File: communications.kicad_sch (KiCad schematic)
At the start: 3 parts, among them J23 Conn_01x90_3Row_Socket

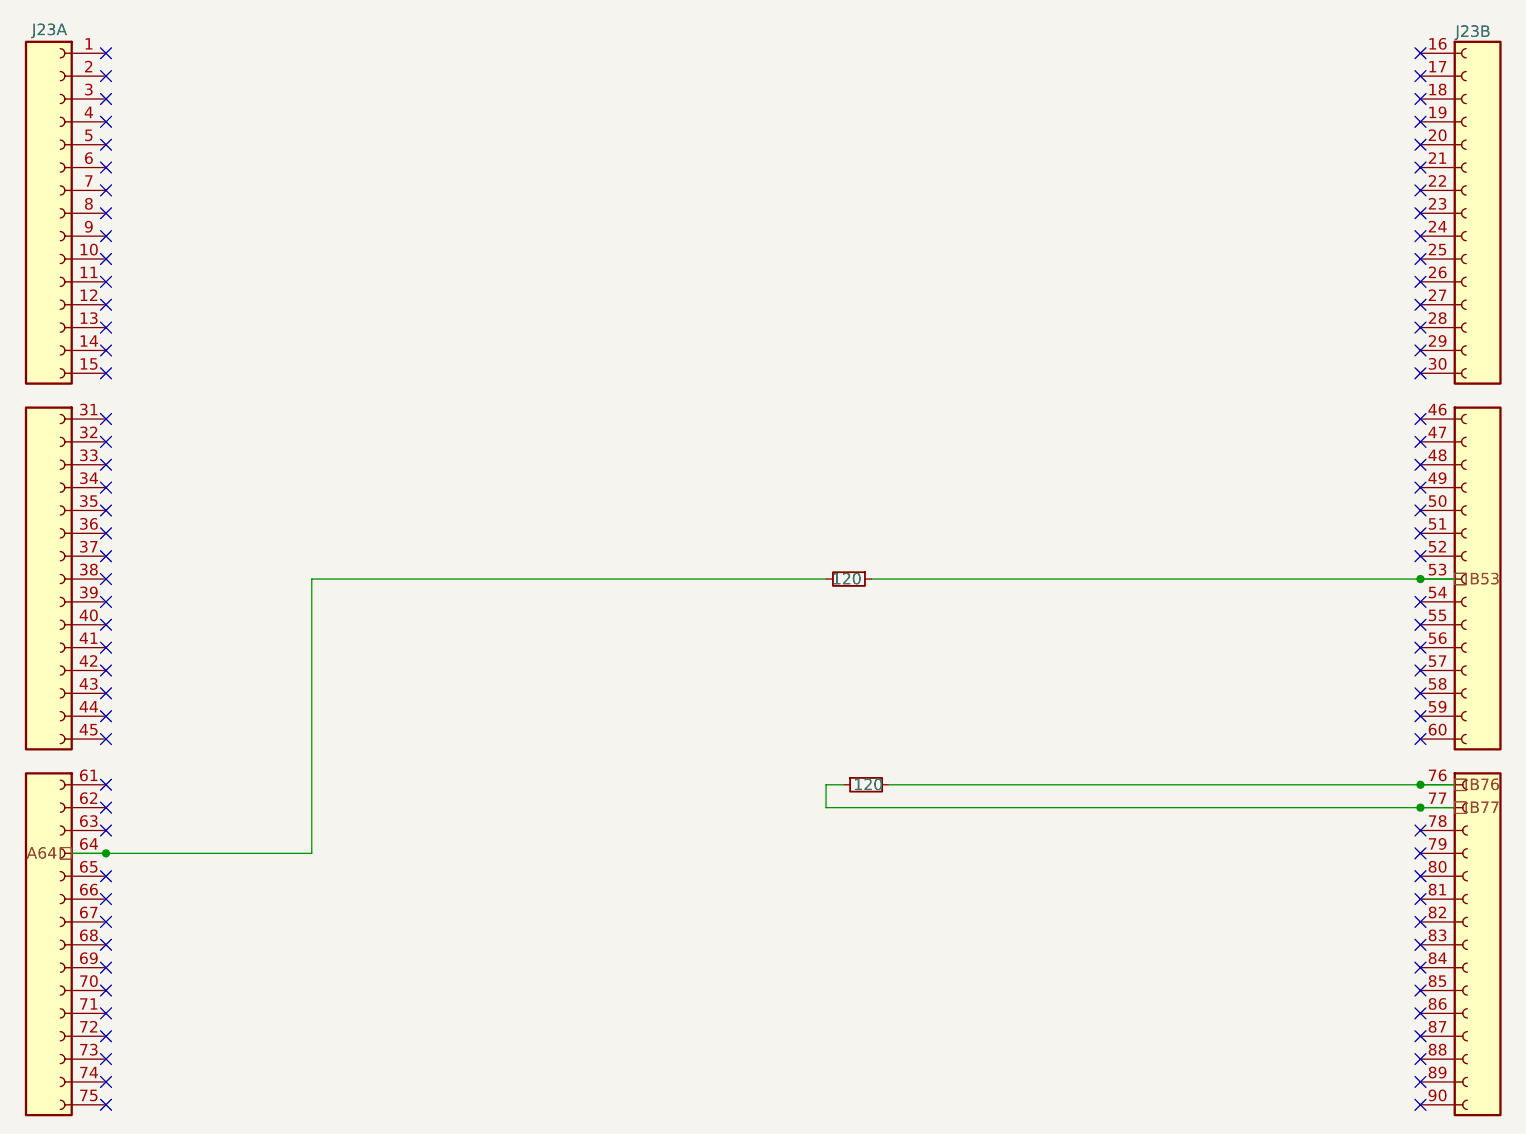
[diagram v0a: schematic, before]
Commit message: external loops
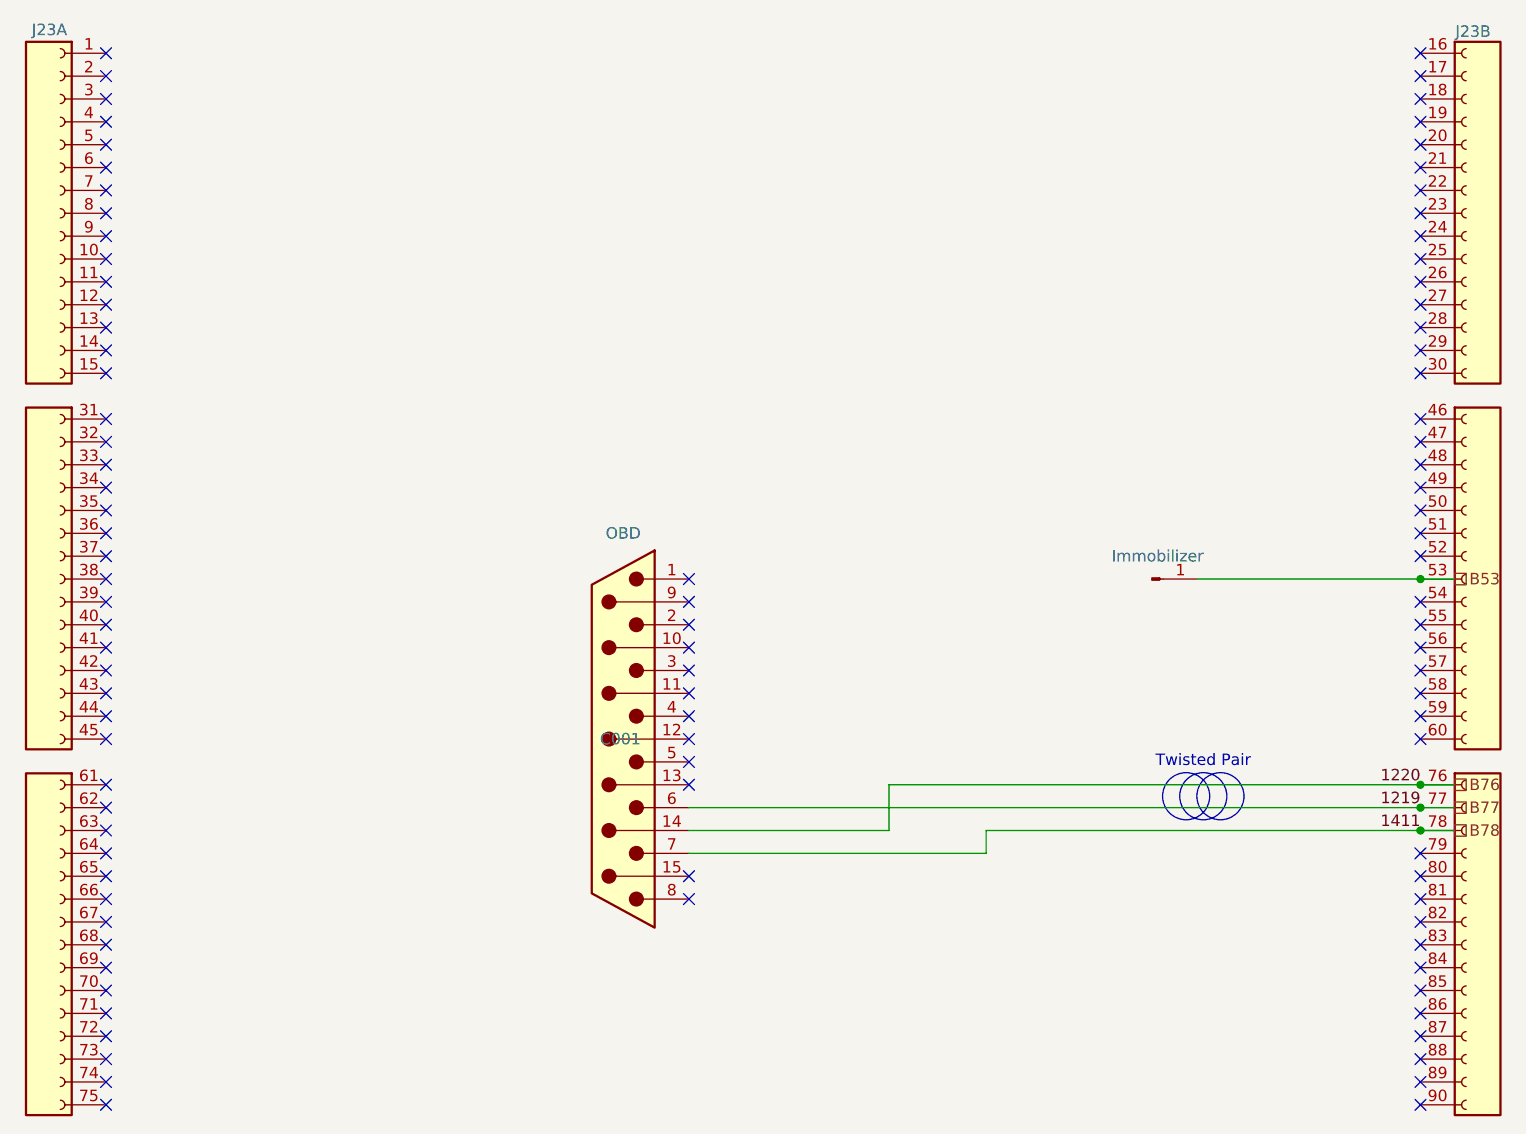
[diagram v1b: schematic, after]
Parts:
- removed R137, R138: 120, Resistor_SMD:R_0603_1608Metric, symbol Device:R_Small
- added J24: OBD, symbol Connector:DA15_Pins
- added J25: Immobilizer, symbol Connector:Conn_01x01_Pin
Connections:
- net B53: now also J25.1 (Pin_1)
- net B76: now also J24.14 (P14)
- net B77: now also J24.6
- net B78: now reaches J23.78 (B78)
- net B78: now also J24.7
- net A64: no longer names the net of J23.64 (A64)
- no-connect marks 86 -> 98
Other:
- note added: "Twisted Pair"
